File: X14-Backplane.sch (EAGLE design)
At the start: 28 parts, among them J2 PXC-PTSM-04-RA-1778641, J3 PXC-8-RA-1778683, J8 PXC-8-RA-1778683

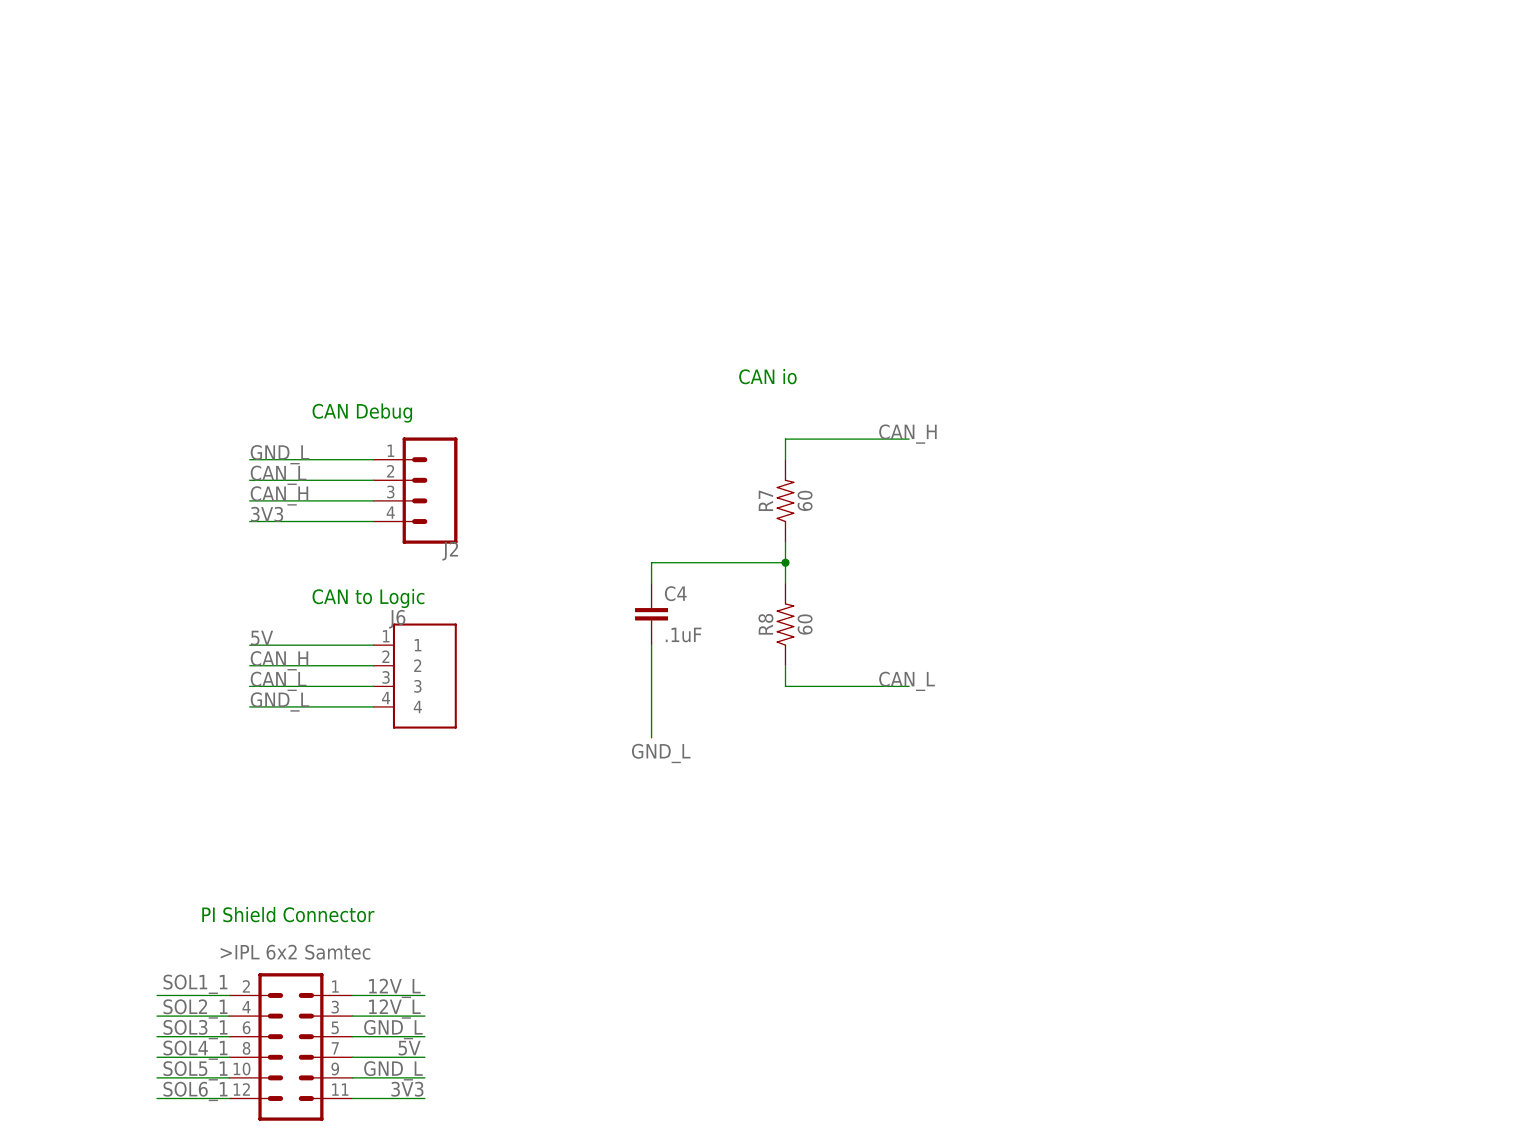
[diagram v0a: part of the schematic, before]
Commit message: X14-Backplane 12/4
This is the most up to date version as of 12/4/2021
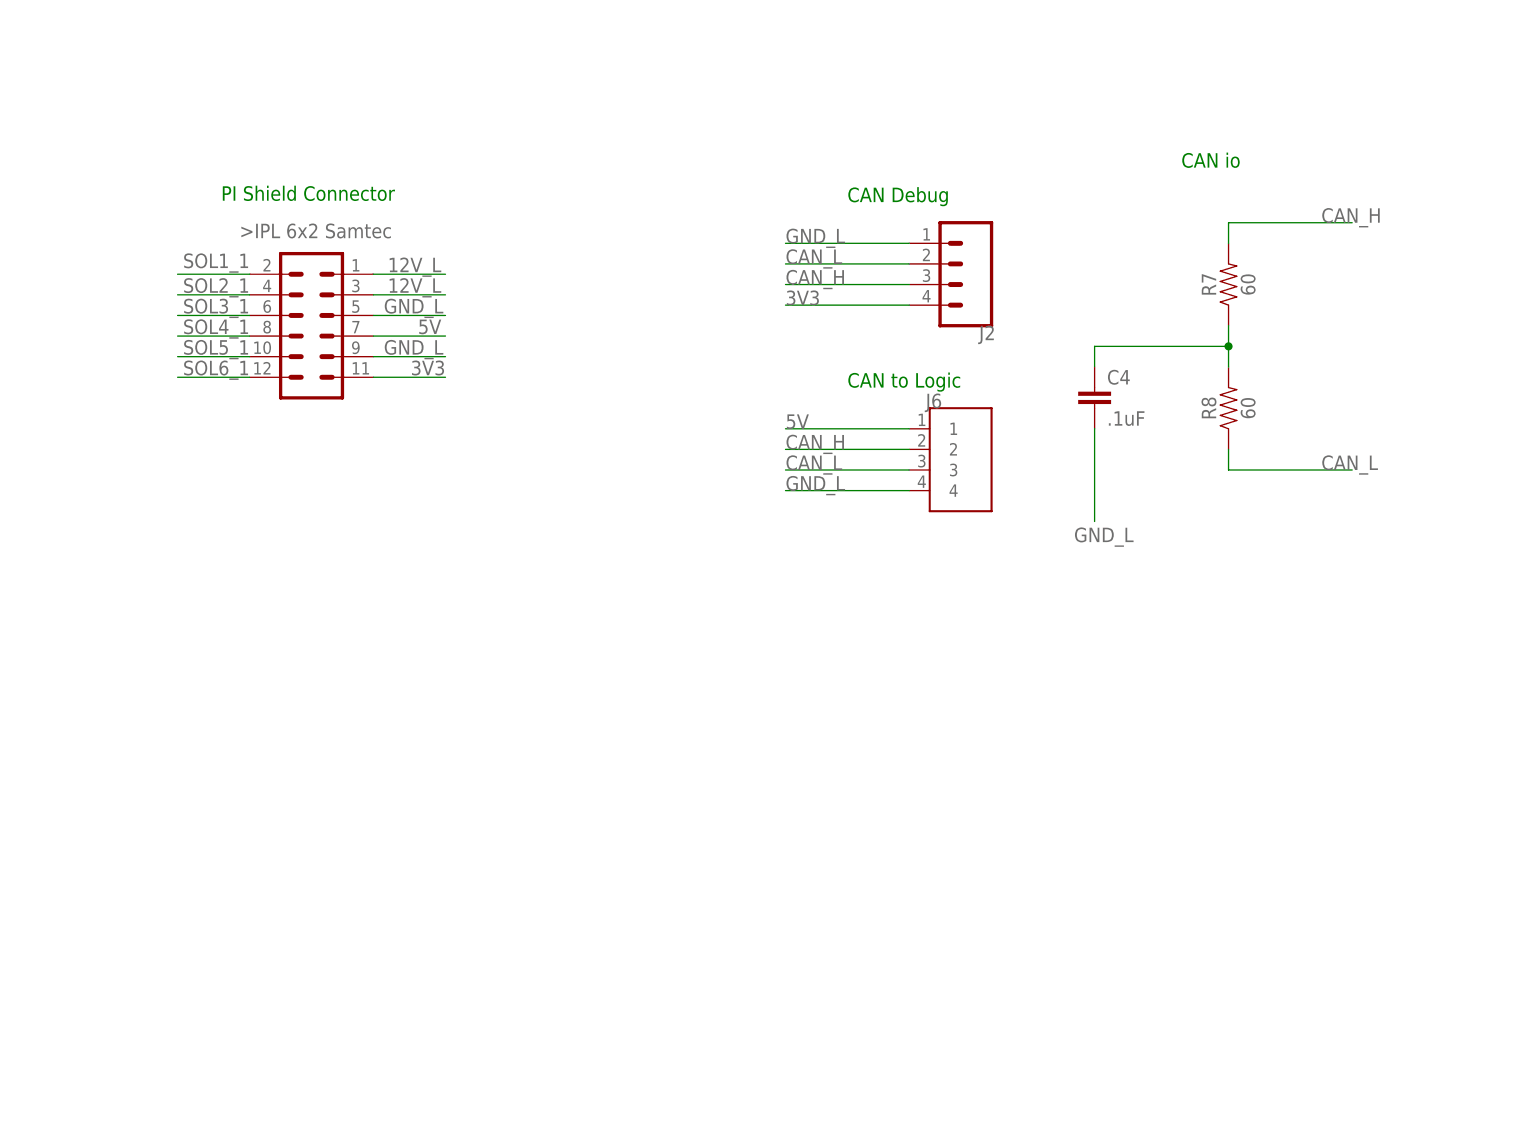
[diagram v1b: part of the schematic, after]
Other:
- moved on the sheet: C4, J2, J6, R7, R8
